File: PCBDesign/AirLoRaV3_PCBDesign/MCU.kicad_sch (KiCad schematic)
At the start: 50 parts, among them IC1 BALFHB-WL-05D3, J2 Conn_Coaxial, SW1 SW_Push, U3 BGS12WN6E6327, U4 STM32WLE5JCIx, Y1 NX2012SA 32.768KHz

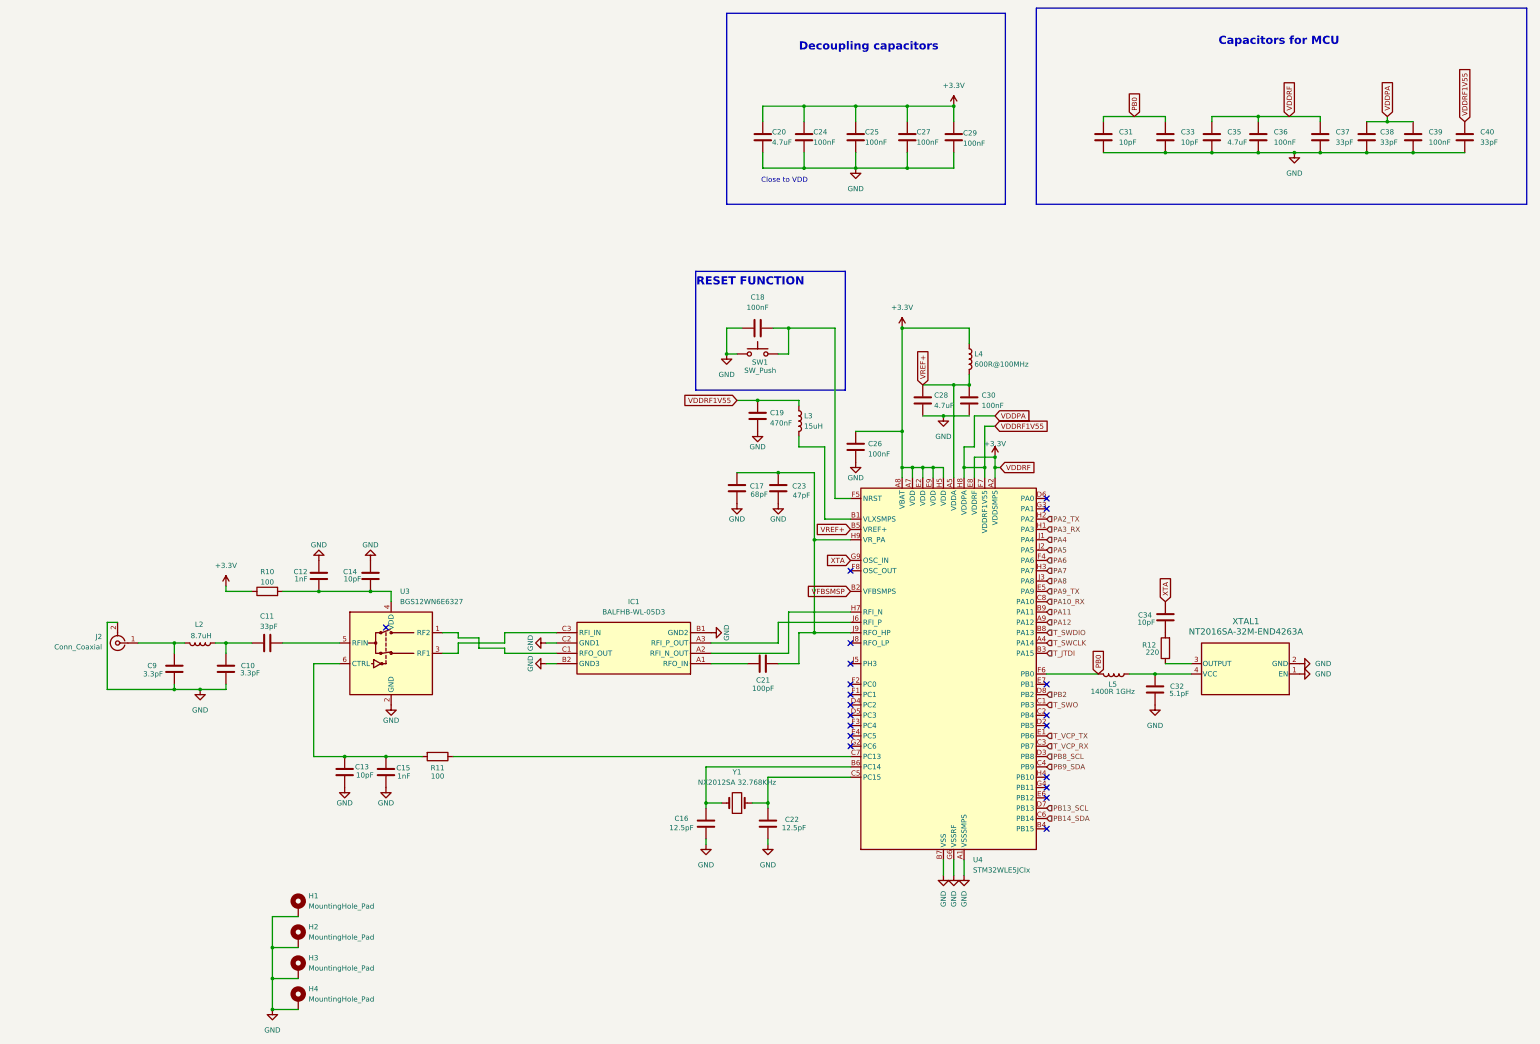
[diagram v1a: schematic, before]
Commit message: Update schematic
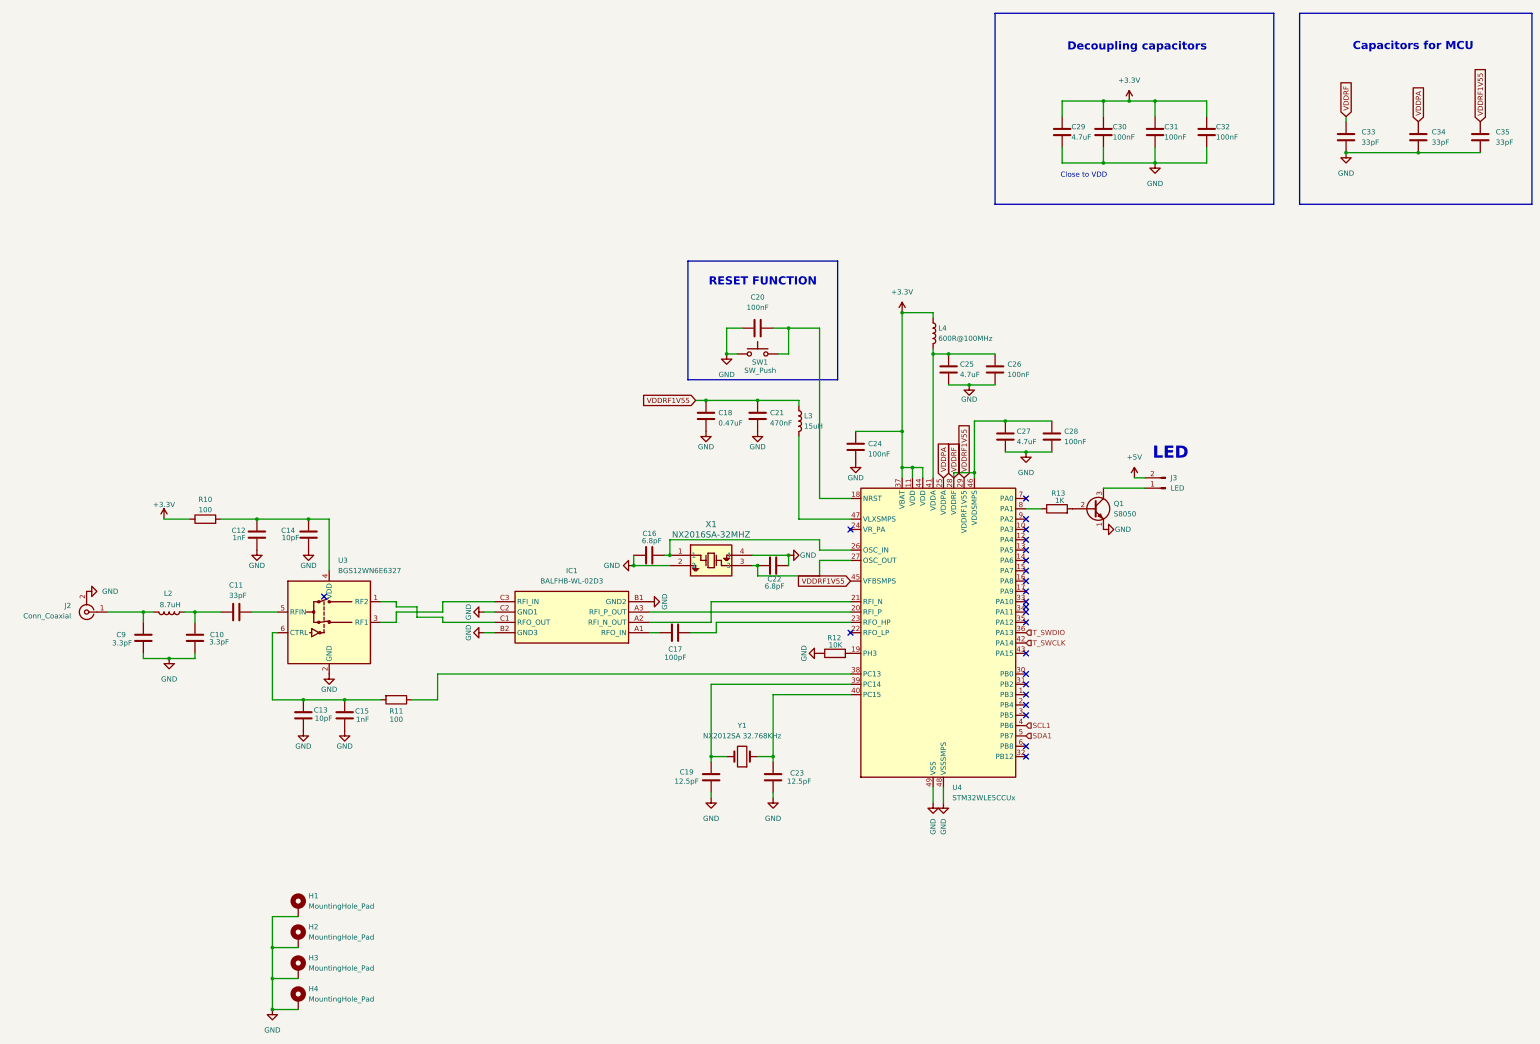
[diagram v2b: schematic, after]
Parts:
- removed C17: 68pF, Capacitor_SMD:C_0603_1608Metric, symbol Device:C
- removed C23: 47pF, Capacitor_SMD:C_0603_1608Metric, symbol Device:C
- removed C29, C36, C39: 100nF, Capacitor_SMD:C_0603_1608Metric, symbol Device:C
- removed C31, C33: 10pF, Capacitor_SMD:C_0603_1608Metric, symbol Device:C
- removed C35: 4.7uF, Capacitor_SMD:C_0603_1608Metric, symbol Device:C
- removed L5: 1400R 1GHz, Inductor_SMD:L_0603_1608Metric, symbol Device:L
- removed U4: STM32WLE5JCIx, Package_BGA:ST_UFBGA-73_5x5mm_Layout9x9_P0.5mm, symbol MCU_ST_STM32WL:STM32WLE5JCIx
- removed XTAL1: NT2016SA-32M-END4263A, footprint:NT2016SA-32M-END4263A_NDK, symbol NT2016SA-32M-:NT2016SA-32M-END4263A
- added C18: 0.47uF, Capacitor_SMD:C_0603_1608Metric, symbol Device:C
- added C27: 4.7uF, Capacitor_SMD:C_0603_1608Metric, symbol Device:C
- added C28: 100nF, Capacitor_SMD:C_0603_1608Metric, symbol Device:C
- added J3: LED, Connector_JST:JST_XA_B02B-XASK-1-A_1x02_P2.50mm_Vertical, symbol Connector:Conn_01x02_Pin
- added Q1: S8050, Package_TO_SOT_SMD:SOT-23, symbol Transistor_BJT:S8050
- added R13: 1K, Resistor_SMD:R_0603_1608Metric, symbol Device:R
- added U4: STM32WLE5CCUx, Package_DFN_QFN:QFN-48-1EP_7x7mm_P0.5mm_EP5.6x5.6mm, symbol MCU_ST_STM32WL:STM32WLE5CCUx
- added X1: NX2016SA-32MHZ, footprint:NX2016SA_NDK, symbol NX2016SA-32MHZ:NX2016SA-32MHZ-EXS00A-CS06654
- C16: renamed from C32; value 5.1pF -> 6.8pF
- C22: renamed from C34; value 10pF -> 6.8pF
- IC1: value BALFHB-WL-05D3 -> BALFHB-WL-02D3
- R12: value 220 -> 10K
- renumbered C21 to C17, C16 to C19, C18 to C20, C19 to C21, C22 to C23, C26 to C24, C28 to C25, C30 to C26, C20 to C29, C24 to C30, C25 to C31, C27 to C32, C37 to C33, C38 to C34, C40 to C35
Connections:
- net XTA is gone; now on net GND: C22.2
- net +3.3V: now also U4.11 (VDD), U4.37 (VBAT), U4.44 (VDD); no longer C33.1
- net GND: now also C12.1, C14.1, R12.1, C18.2, C27.2, C28.2, Q1.1 (E), U4.48 (VSSSMPS), U4.49 (VSS), X1.2, X1.4; no longer C12.2, C14.2
- net T_SWCLK: now also U4.42 (PA14)
- net T_SWDIO: now also U4.36 (PA13)
- net VDDPA: now also U4.25 (VDDPA); no longer C21.1, C35.1, L3.1
- net at IC1.A2 (RFI_N_OUT): now also U4.21 (RFI_N)
- net at IC1.A3 (RFI_P_OUT): now also U4.20 (RFI_P)
- net at C16.2: now also U4.26 (OSC_IN), X1.1
- net at R11.1: now also U4.38 (PC13)
- net at C23.2, Y1.1: now also U4.40 (PC15)
- net at C19.2, Y1.2: now also U4.39 (PC14)
- net at R10.2, U3.4 (VDD): now also C12.2, C14.2; no longer C12.1, C14.1
- net at C22.1: now also U4.27 (OSC_OUT), X1.3; no longer R12.2
- net at C17.2: now also U4.23 (RFO_HP)
- net at C20.2, SW1.2: now also U4.18 (NRST)
- net at L3.2: now also U4.47 (VLXSMPS)
- net VREF+: no longer names the net of C25.1, C26.1, L4.2
- net VREF+: now also U4.41 (VDDA)
- new net: R12.2, U4.19 (PH3)
- new net: R13.1, U4.8 (PA1)
- new net: J3.1 (Pin_1), Q1.3 (C)
- new net: Q1.2 (B), R13.2
- new net +5V: J3.2 (Pin_2)
- new net SCL1: U4.4 (PB6)
- new net SDA1: U4.5 (PB7)
- new net VDDRF: C27.1, C28.1, C33.1, U4.28 (VDDRF), U4.46 (VDDSMPS)
- new net VDDRF1V55: C18.1, C21.1, C35.1, L3.1, U4.29 (VDDRF1V55), U4.45 (VFBSMPS)
- no-connect marks 20 -> 24
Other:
- note added: "LED"
- moved on the sheet: C10, C11, C12, C13, C14, C15, C16, C17, C19, C22, C23, C25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
